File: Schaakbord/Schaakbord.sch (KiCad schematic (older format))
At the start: 65 parts, among them IC1 ZLDO1117K33TC, IC10 AH3572-SA-7, IC11 MAX6955AAX+, IC12 SN74LVC2T45DCTRE4, IC13 M24C04-RMN6TP, IC2 SN74HC165DR, IC3 AH3572-SA-7, IC4 AH3572-SA-7, IC5 AH3572-SA-7, IC6 AH3572-SA-7, IC7 AH3572-SA-7, IC8 AH3572-SA-7, IC9 AH3572-SA-7, J1 Conn_01x02, J2 Conn_01x06, J3 Conn_01x04, J4 Conn_01x03, J5 Conn_01x03, J6 Conn_01x04, J7 Conn_01x04, SW1 SW_Push, SW2 SW_Push, U2 STM32F101RDTx

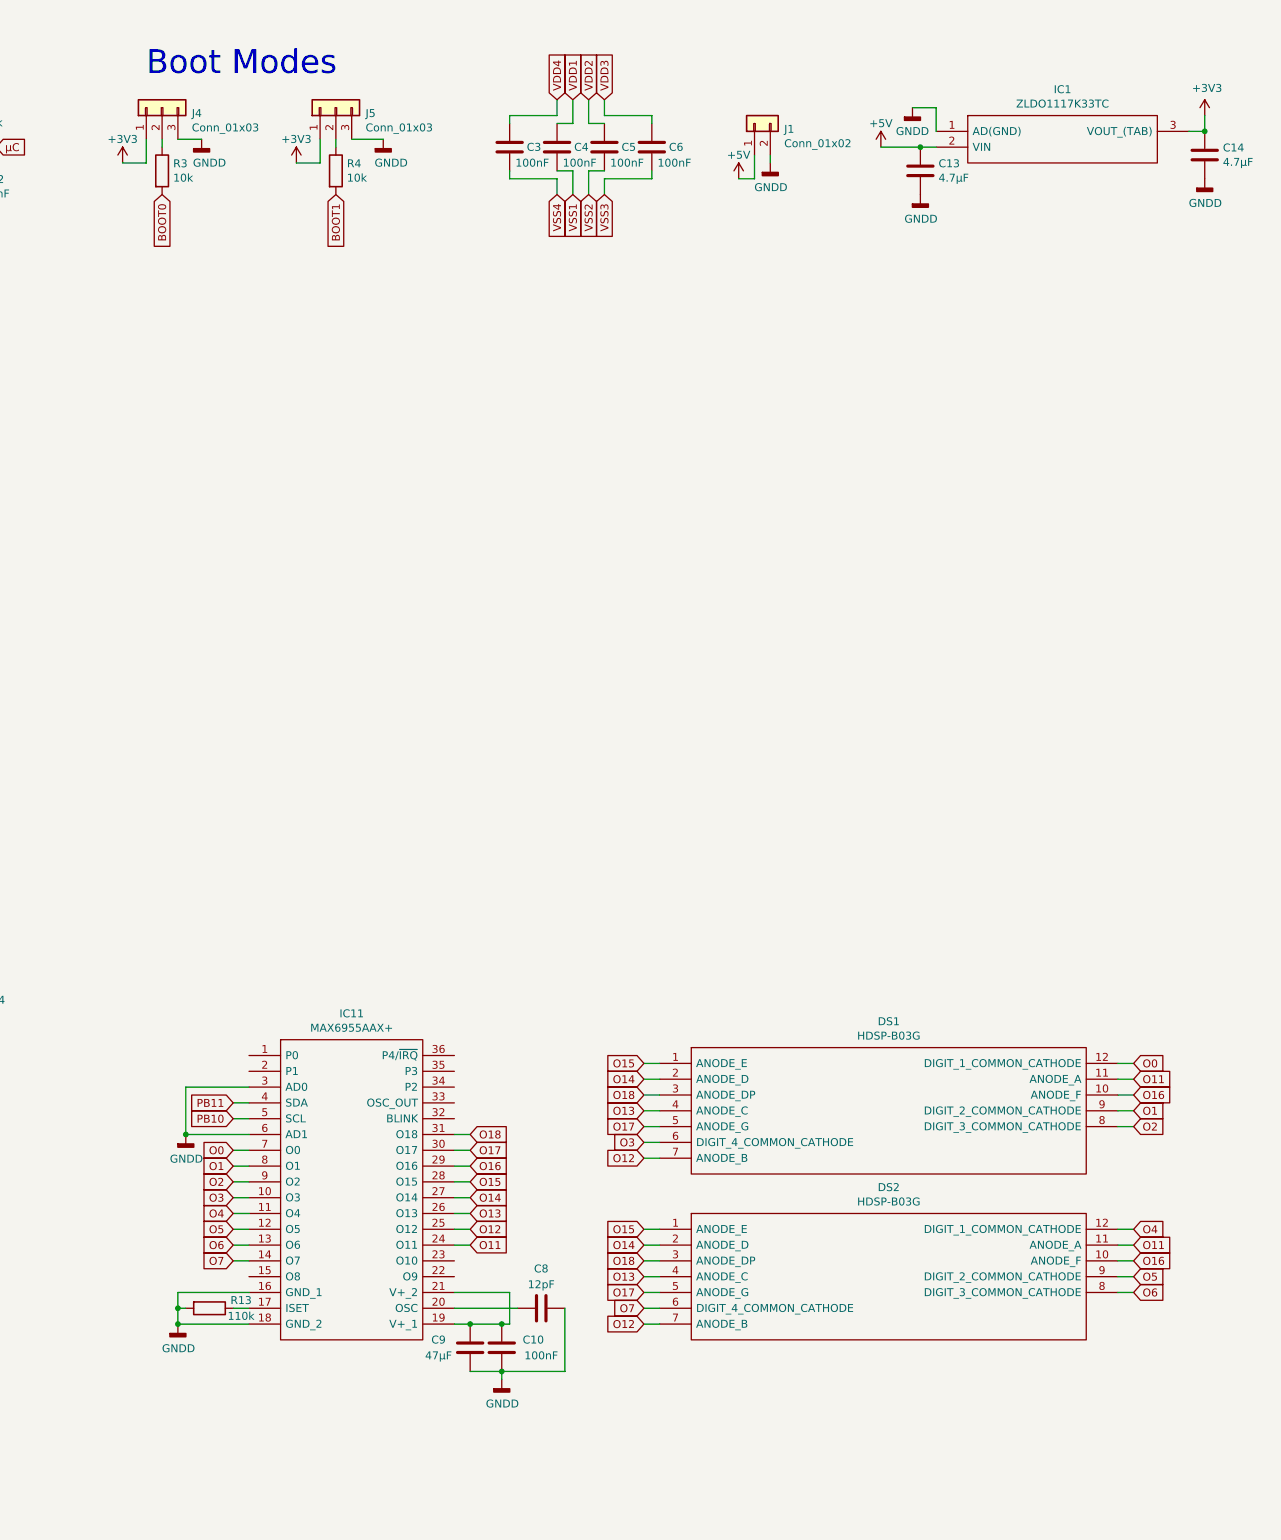
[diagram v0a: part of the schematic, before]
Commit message: Schematic Update
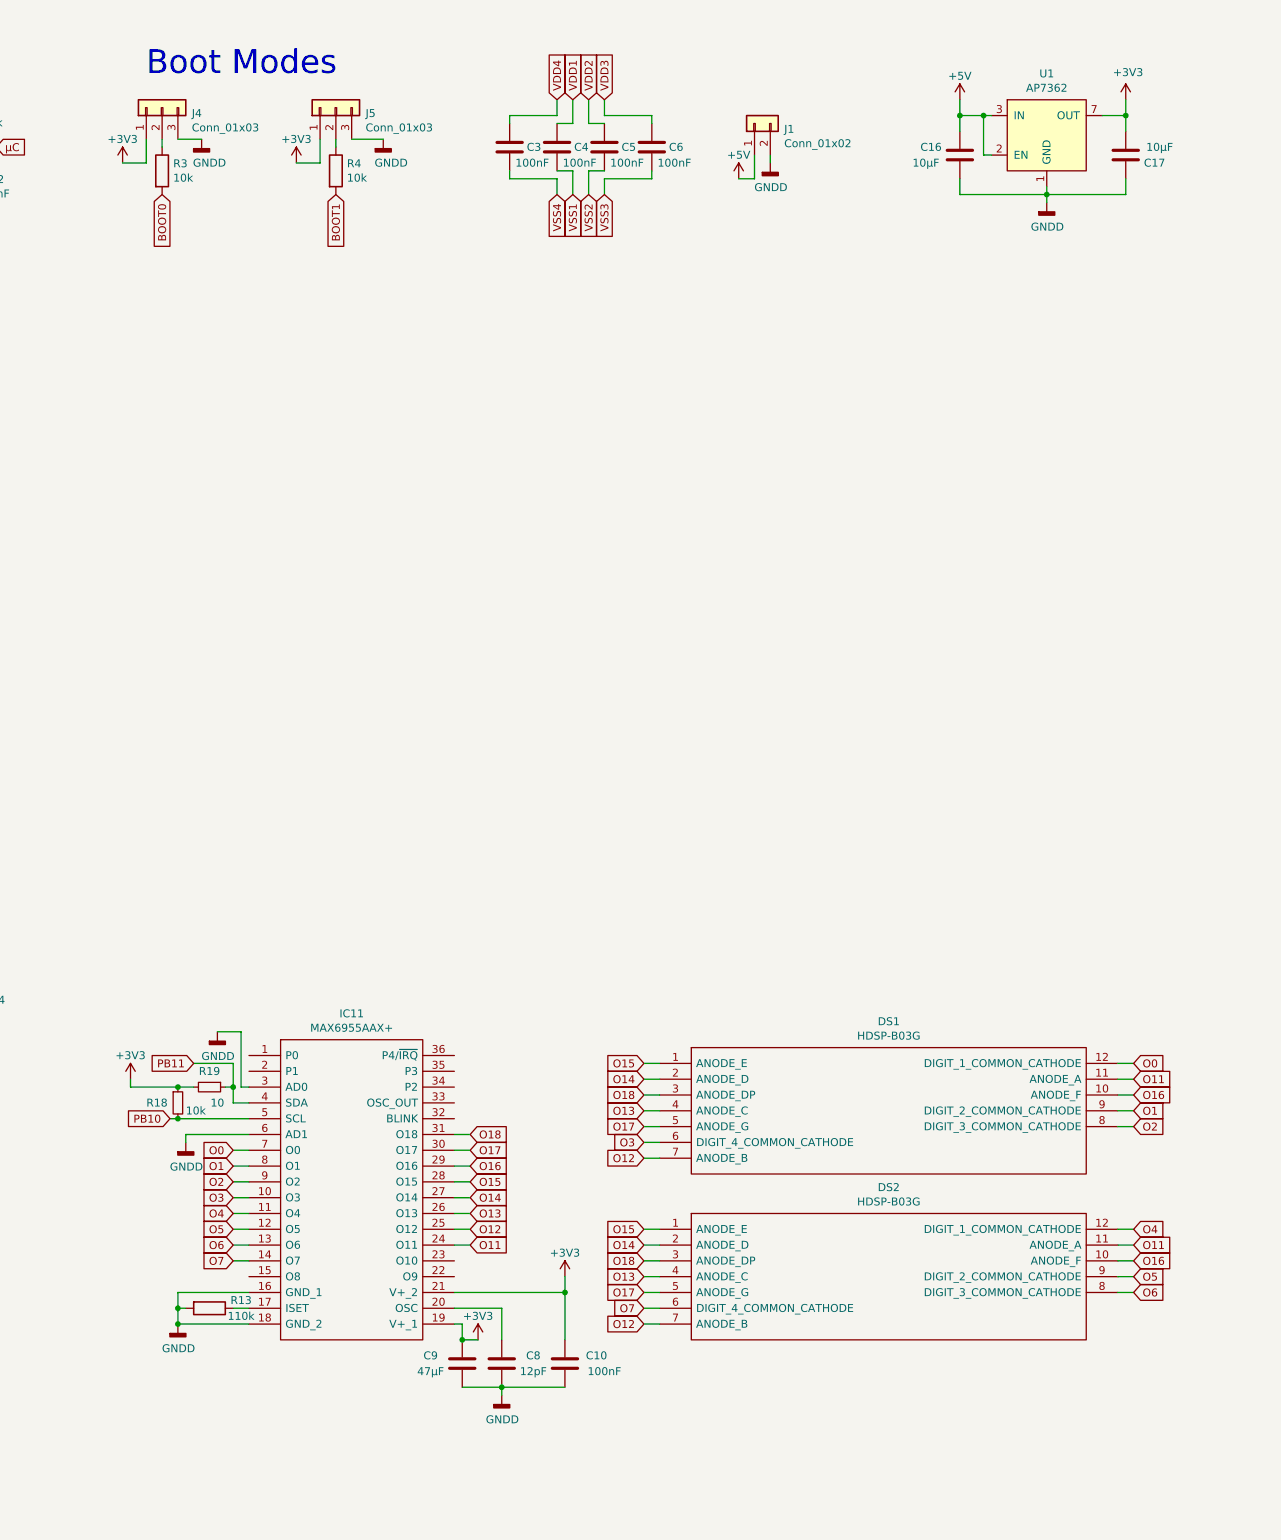
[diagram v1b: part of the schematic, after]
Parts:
- removed C13, C14: 4.7µF, symbol Device:C
- removed IC1: ZLDO1117K33TC, TO-252_1, symbol SamacSys_Parts:ZLDO1117K33TC
- added C16, C17: 10µF, symbol Device:C
- added R18: 10k, symbol Device:R_Small
- added R19: 10, symbol Device:R_Small
- added U1: AP7362, Package_SO:Diodes_SO-8EP, symbol SamacSys_Parts:AP7362
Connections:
- net +3V3: now also C10.1, C9.2, IC11.19 (V+_1), IC11.21 (V+_2), C17.1, R18.1, R19.2, U1.5 (OUT), U1.6 (OUT), U1.7 (OUT)
- net +5V: now also C16.2, U1.2 (EN), U1.3 (IN), U1.4 (IN)
- net PB10: now also R18.2
- net PB11: now also R19.1
- net GNDD renamed GND
- net GND: now also C16.1, C17.2, U1.1 (GND), U1.9 (GND)
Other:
- moved on the sheet: C10, C8, C9
